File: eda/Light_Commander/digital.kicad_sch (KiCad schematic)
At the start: 1 part, among them U1 STM32F446RETx

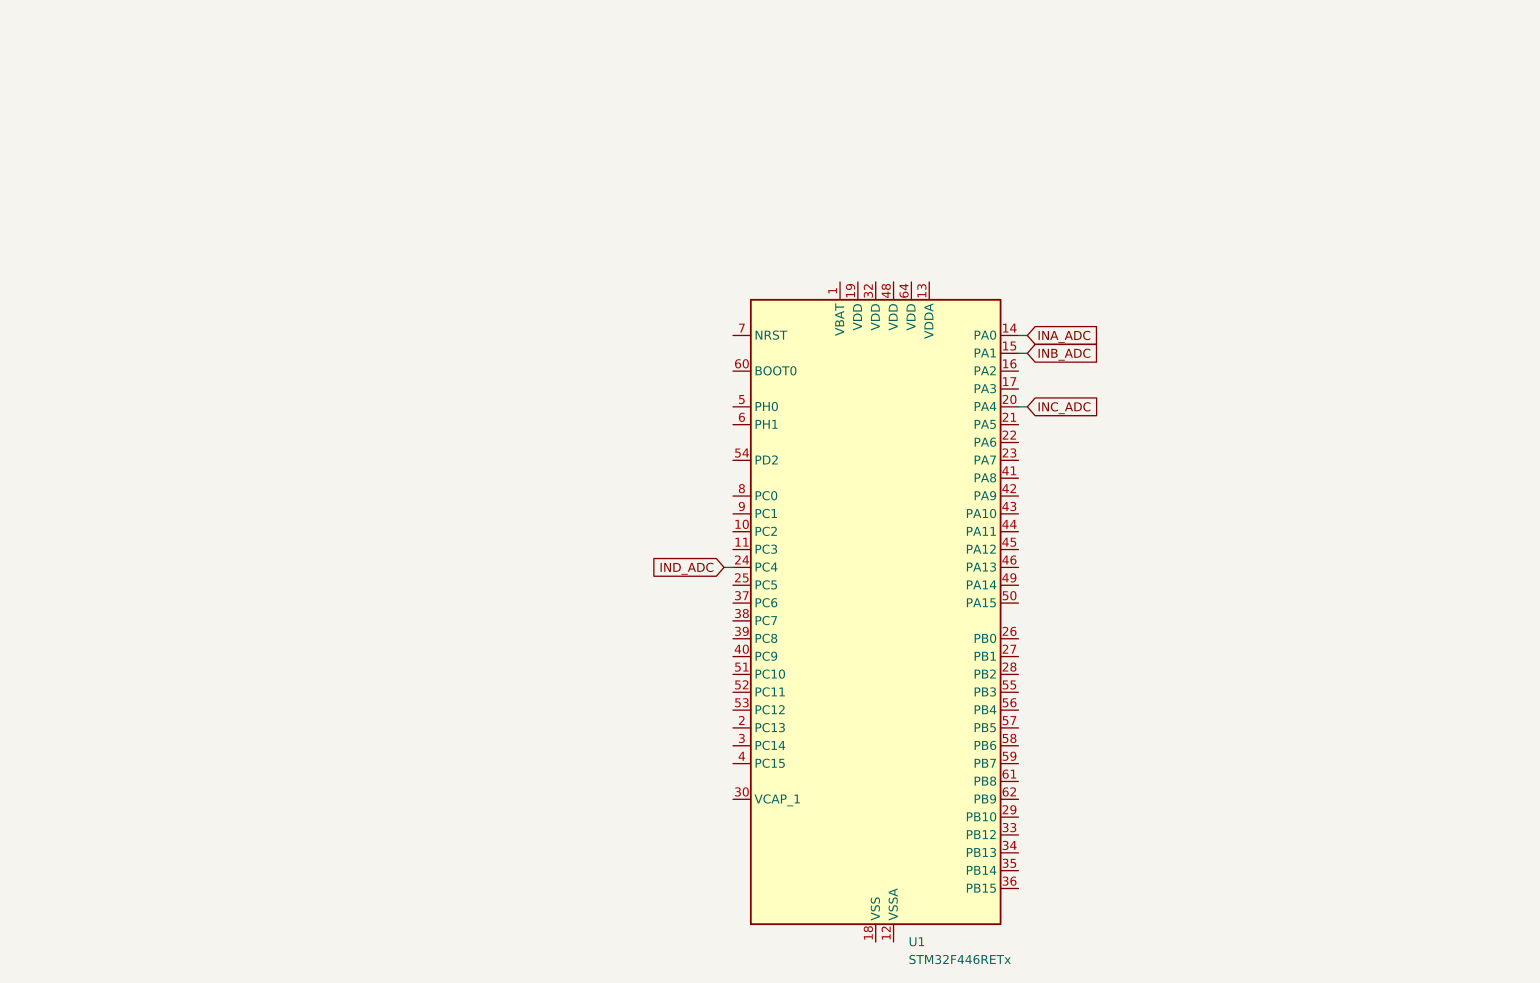
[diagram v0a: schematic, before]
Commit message: Power and UI on PCB
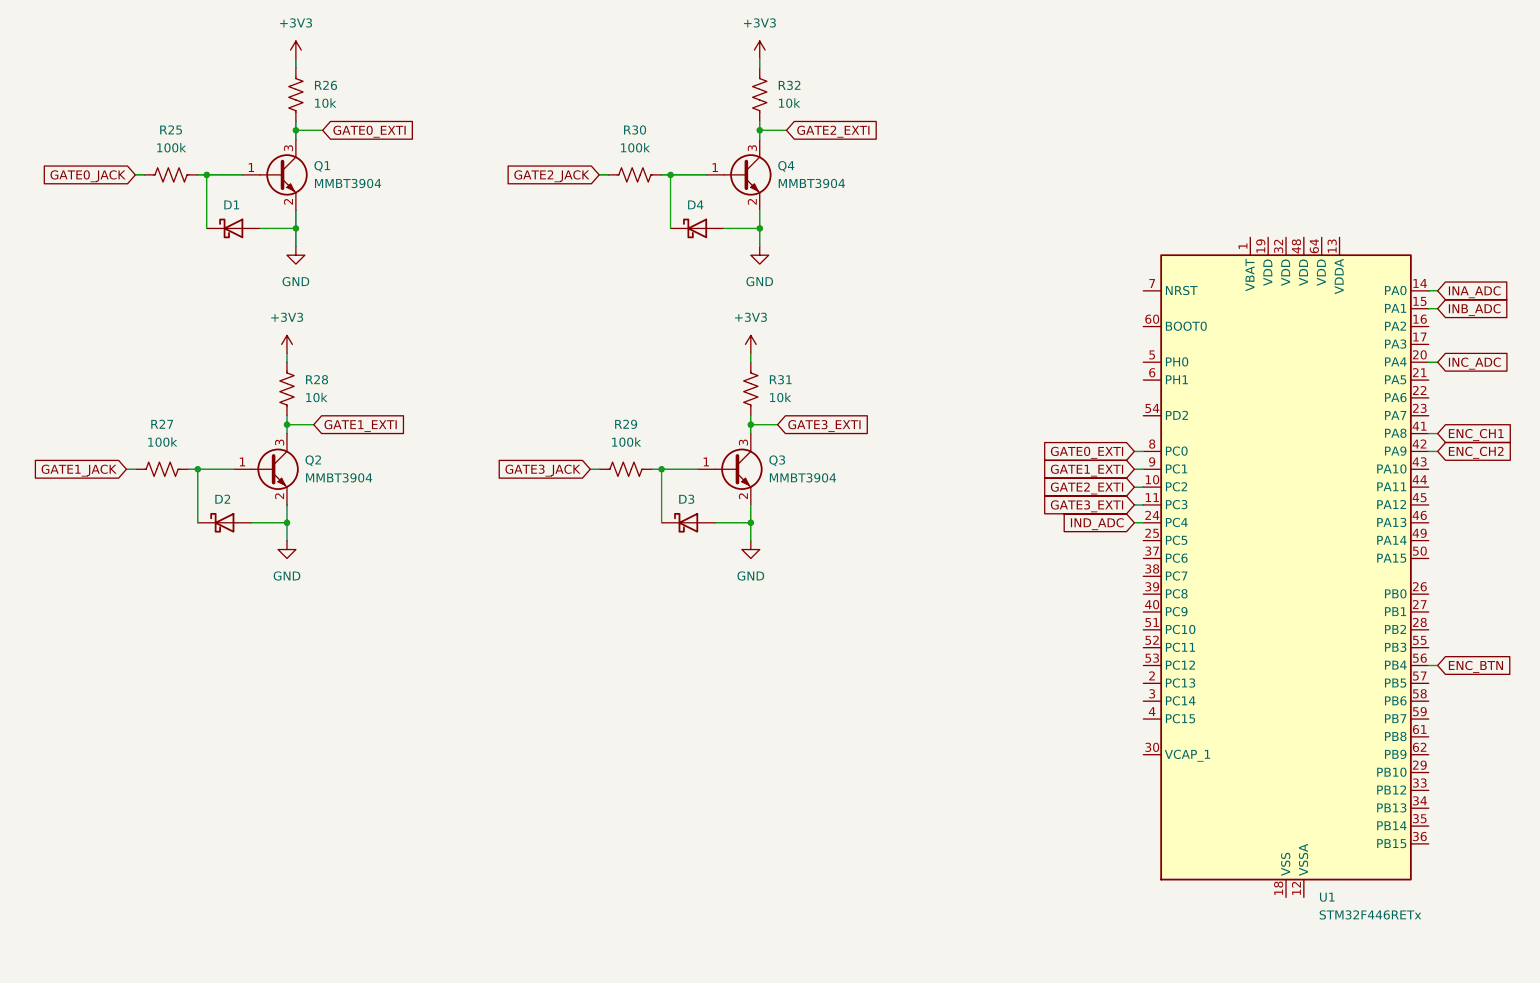
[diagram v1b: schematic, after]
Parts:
- added D1, D2, D3, D4: GSBAT54W, Diode_SMD:D_SOD-123, symbol Device:D_Schottky
- added Q1, Q2, Q3, Q4: MMBT3904, Package_TO_SOT_SMD:SOT-23, symbol Transistor_BJT:MMBT3904
- added R25, R27, R29, R30: 100k, Resistor_SMD:R_0805_2012Metric, symbol Device:R_US
- added R26, R28, R31, R32: 10k, Resistor_SMD:R_0805_2012Metric, symbol Device:R_US
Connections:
- net GATE2_EXTI: now reaches U1.10 (PC2)
- net GATE2_EXTI: now also Q4.3 (C), R32.2
- net GATE3_EXTI: now reaches U1.11 (PC3)
- net GATE3_EXTI: now also Q3.3 (C), R31.2
- net ENC_CH1: now reaches U1.41 (PA8)
- net ENC_CH2: now reaches U1.42 (PA9)
- net ENC_BTN: now reaches U1.56 (PB4)
- net GATE0_EXTI: now reaches U1.8 (PC0)
- net GATE0_EXTI: now also Q1.3 (C), R26.2
- net GATE1_EXTI: now reaches U1.9 (PC1)
- net GATE1_EXTI: now also Q2.3 (C), R28.2
- new net: D1.1 (K), Q1.1 (B), R25.2
- new net: D4.1 (K), Q4.1 (B), R30.2
- new net: D2.1 (K), Q2.1 (B), R27.2
- new net: D3.1 (K), Q3.1 (B), R29.2
- new net +3V3: R26.1, R28.1, R31.1, R32.1
- new net GATE0_JACK: R25.1
- new net GATE1_JACK: R27.1
- new net GATE2_JACK: R30.1
- new net GATE3_JACK: R29.1
- new net GND: D1.2 (A), D2.2 (A), D3.2 (A), D4.2 (A), Q1.2 (E), Q2.2 (E), Q3.2 (E), Q4.2 (E)
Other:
- moved on the sheet: U1
